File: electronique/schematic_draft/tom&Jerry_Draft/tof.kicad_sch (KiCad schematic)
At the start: 3 parts, among them U701 VL53L1CXV0FY1

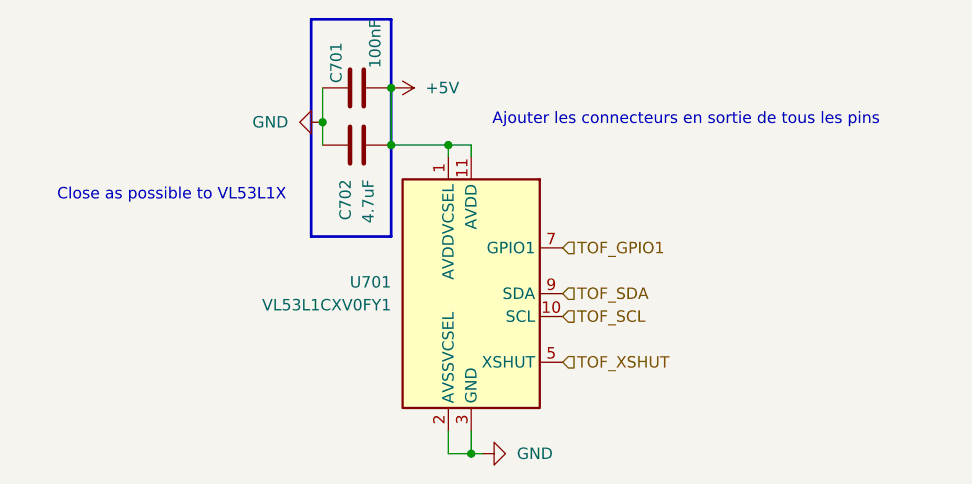
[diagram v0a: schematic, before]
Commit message: KiCAD V3 - 18.09.2024
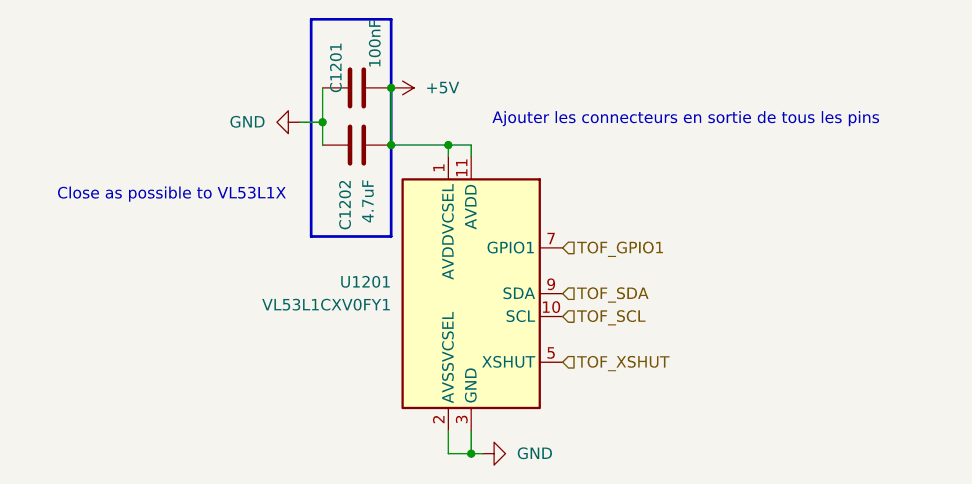
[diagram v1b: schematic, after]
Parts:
- renumbered C701 to C1201, C702 to C1202, U701 to U1201
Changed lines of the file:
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@@
+	(wire
+		(pts
+			(xy 119.38 69.85) (xy 121.92 69.85)
+		)
+		(stroke
+			(width 0)
+			(type default)
+		)
+	)
 	(wire
 		(pts
@@
 		(dnp no)
 		(fields_autoplaced yes)
-		(property "Reference" "C702"
+		(property "Reference" "C1202"
 			(at 124.4599 76.2 0)
 			(effects
@@
 	(symbol
 		(lib_id "power:GND")
-		(at 121.92 69.85 270)
+		(at 119.38 69.85 270)
 		(mirror x)
 		(unit 1)
@@
 		(dnp no)
 		(fields_autoplaced yes)
-		(property "Reference" "#PWR0702"
-			(at 115.57 69.85 0)
+		(property "Reference" "#PWR01202"
+			(at 113.03 69.85 0)
 			(effects
 				(font
@@
 		)
 		(property "Value" "GND"
-			(at 118.11 69.8499 90)
+			(at 115.57 69.8499 90)
 			(effects
 				(font
@@
 		)
 		(property "Footprint" ""
-			(at 121.92 69.85 0)
+			(at 119.38 69.85 0)
 			(effects
 				(font
@@
 		)
 		(property "Datasheet" ""
-			(at 121.92 69.85 0)
+			(at 119.38 69.85 0)
 			(effects
 				(font
@@
 		)
 		(property "Description" "Power symbol creates a global label with name \"GND\" , ground"
-			(at 121.92 69.85 0)
+			(at 119.38 69.85 0)
 			(effects
 				(font
@@
 		(dnp no)
 		(fields_autoplaced yes)
-		(property "Reference" "#PWR0701"
+		(property "Reference" "#PWR01201"
 			(at 125.73 66.04 0)
 			(effects
@@
 		(on_board yes)
 		(dnp no)
-		(property "Reference" "C701"
+		(property "Reference" "C1201"
 			(at 123.444 60.96 0)
 			(effects
@@
 		(dnp no)
 		(fields_autoplaced yes)
-		(property "Reference" "#PWR0703"
+		(property "Reference" "#PWR01203"
 			(at 146.05 106.68 0)
 			(effects
@@
 		(dnp no)
 		(fields_autoplaced yes)
-		(property "Reference" "U701"
+		(property "Reference" "U1201"
 			(at 129.54 87.6299 0)
 			(effects
